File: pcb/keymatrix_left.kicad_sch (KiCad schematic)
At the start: 42 parts, among them SW10 SW_Push, SW11 SW_Push, SW12 SW_Push, SW13 SW_Push, SW14 SW_Push, SW15 SW_Push, SW16 SW_Push, SW17 SW_Push, SW18 SW_Push, SW19 SW_Push, SW2 SW_Push, SW20 SW_Push, SW21 SW_Push, SW22 SW_Push, SW3 SW_Push, SW4 SW_Push, SW5 SW_Push, SW6 SW_Push, SW7 SW_Push, SW8 SW_Push, SW9 SW_Push

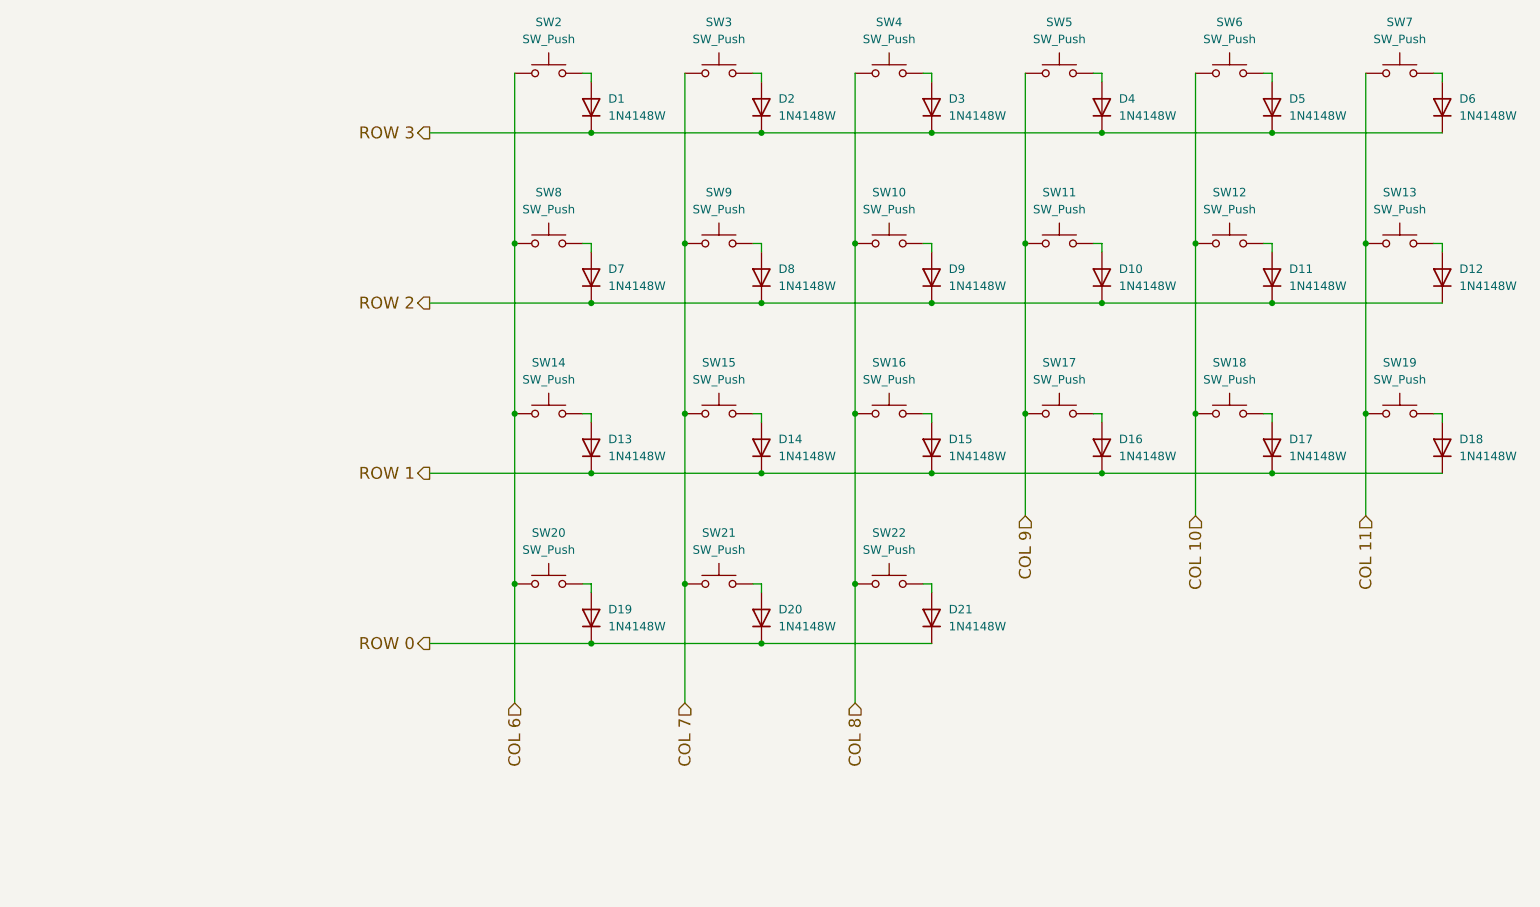
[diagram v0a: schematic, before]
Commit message: update everything
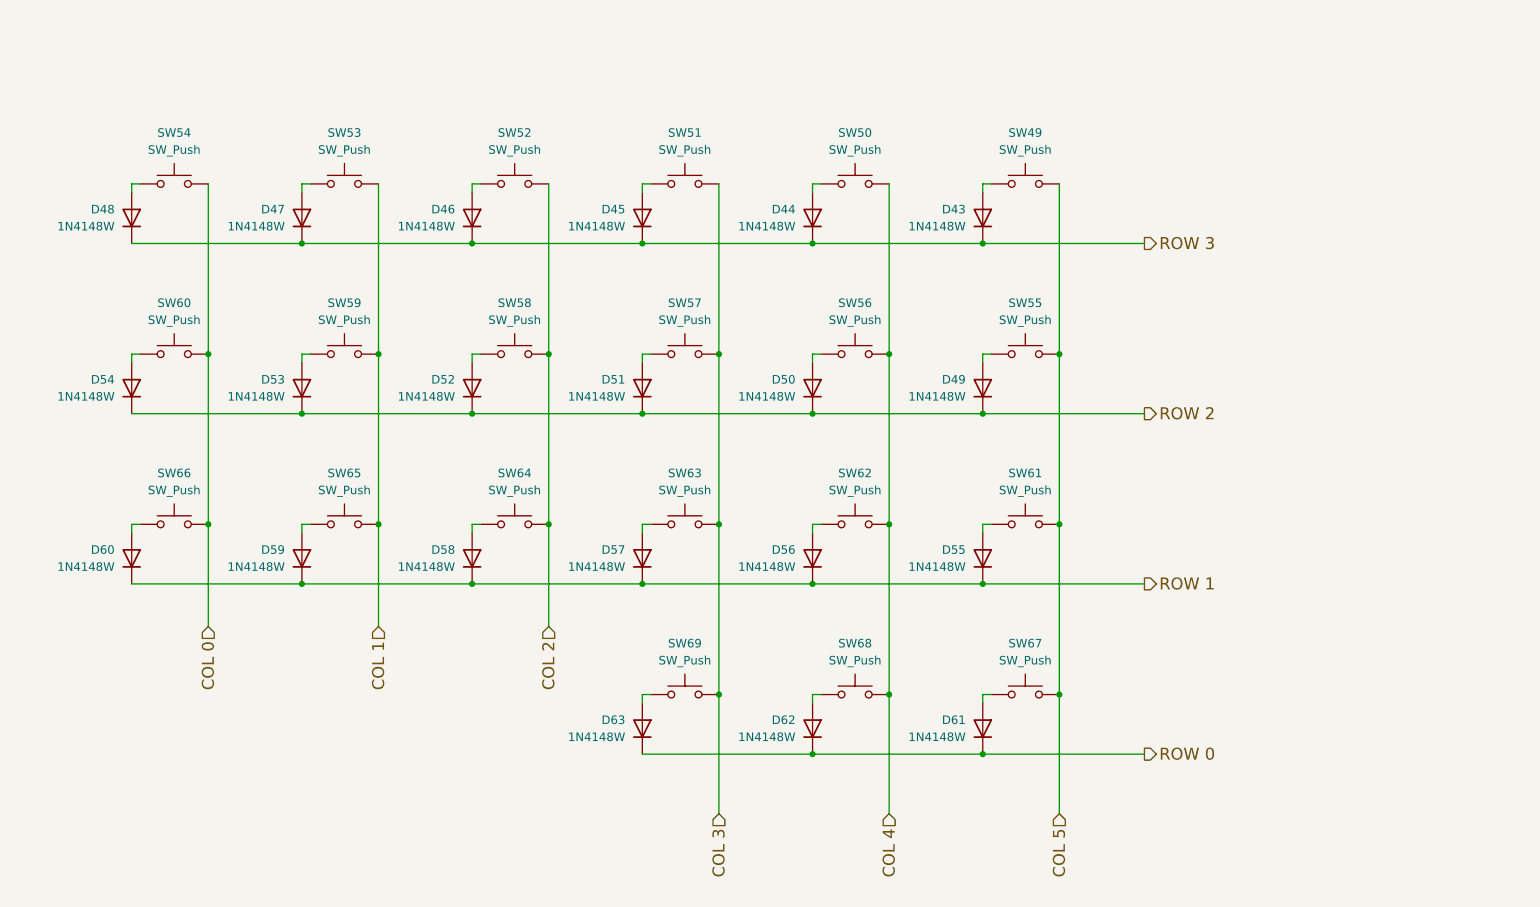
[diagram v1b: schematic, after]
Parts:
- removed D1, D10, D11, D12, D13, D14, D15, D16, D17, D18, D19, D2, D20, D21, D3, D4, D5, D6, D7, D8, D9: 1N4148W, Diode_SMD:D_SOD-123, symbol Diode:1N4148W
- removed SW10, SW11, SW12, SW13, SW14, SW15, SW16, SW17, SW18, SW19, SW2, SW20, SW21, SW22, SW3, SW4, SW5, SW6, SW7, SW8, SW9: SW_Push, kbd:keyswitch_choc12_hotswap_1u, symbol Switch:SW_Push
- added D43, D44, D45, D46, D47, D48, D49, D50, D51, D52, D53, D54, D55, D56, D57, D58, D59, D60, D61, D62, D63: 1N4148W, Diode_SMD:D_SOD-123, symbol Diode:1N4148W
- added SW49, SW50, SW51, SW52, SW53, SW54, SW55, SW56, SW57, SW58, SW59, SW60, SW61, SW62, SW63, SW64, SW65, SW66, SW67, SW68, SW69: SW_Push, kbd:keyswitch_choc12_hotswap_1u, symbol Switch:SW_Push
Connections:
- net ROW 0: now also D61.1 (K), D62.1 (K), D63.1 (K)
- net ROW 1: now also D55.1 (K), D56.1 (K), D57.1 (K), D58.1 (K), D59.1 (K), D60.1 (K)
- net ROW 2: now also D49.1 (K), D50.1 (K), D51.1 (K), D52.1 (K), D53.1 (K), D54.1 (K)
- net ROW 3: now also D43.1 (K), D44.1 (K), D45.1 (K), D46.1 (K), D47.1 (K), D48.1 (K)
- new net: D59.2 (A), SW65.2
- new net: D57.2 (A), SW63.2
- new net: D49.2 (A), SW55.2
- new net: D54.2 (A), SW60.2
- new net: D58.2 (A), SW64.2
- new net: D51.2 (A), SW57.2
- new net: D45.2 (A), SW51.2
- new net: D48.2 (A), SW54.2
- new net: D50.2 (A), SW56.2
- new net: D63.2 (A), SW69.2
- new net: D60.2 (A), SW66.2
- new net: D46.2 (A), SW52.2
- new net: D52.2 (A), SW58.2
- new net: D56.2 (A), SW62.2
- new net: D44.2 (A), SW50.2
- new net: D55.2 (A), SW61.2
- new net: D61.2 (A), SW67.2
- new net: D43.2 (A), SW49.2
- new net: D62.2 (A), SW68.2
- new net: D47.2 (A), SW53.2
- new net: D53.2 (A), SW59.2
- new net COL 0: SW54.1, SW60.1, SW66.1
- new net COL 1: SW53.1, SW59.1, SW65.1
- new net COL 2: SW52.1, SW58.1, SW64.1
- new net COL 3: SW51.1, SW57.1, SW63.1, SW69.1
- new net COL 4: SW50.1, SW56.1, SW62.1, SW68.1
- new net COL 5: SW49.1, SW55.1, SW61.1, SW67.1
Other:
- company: (none) -> Dylan DiBeneditto

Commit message: finished routing second half
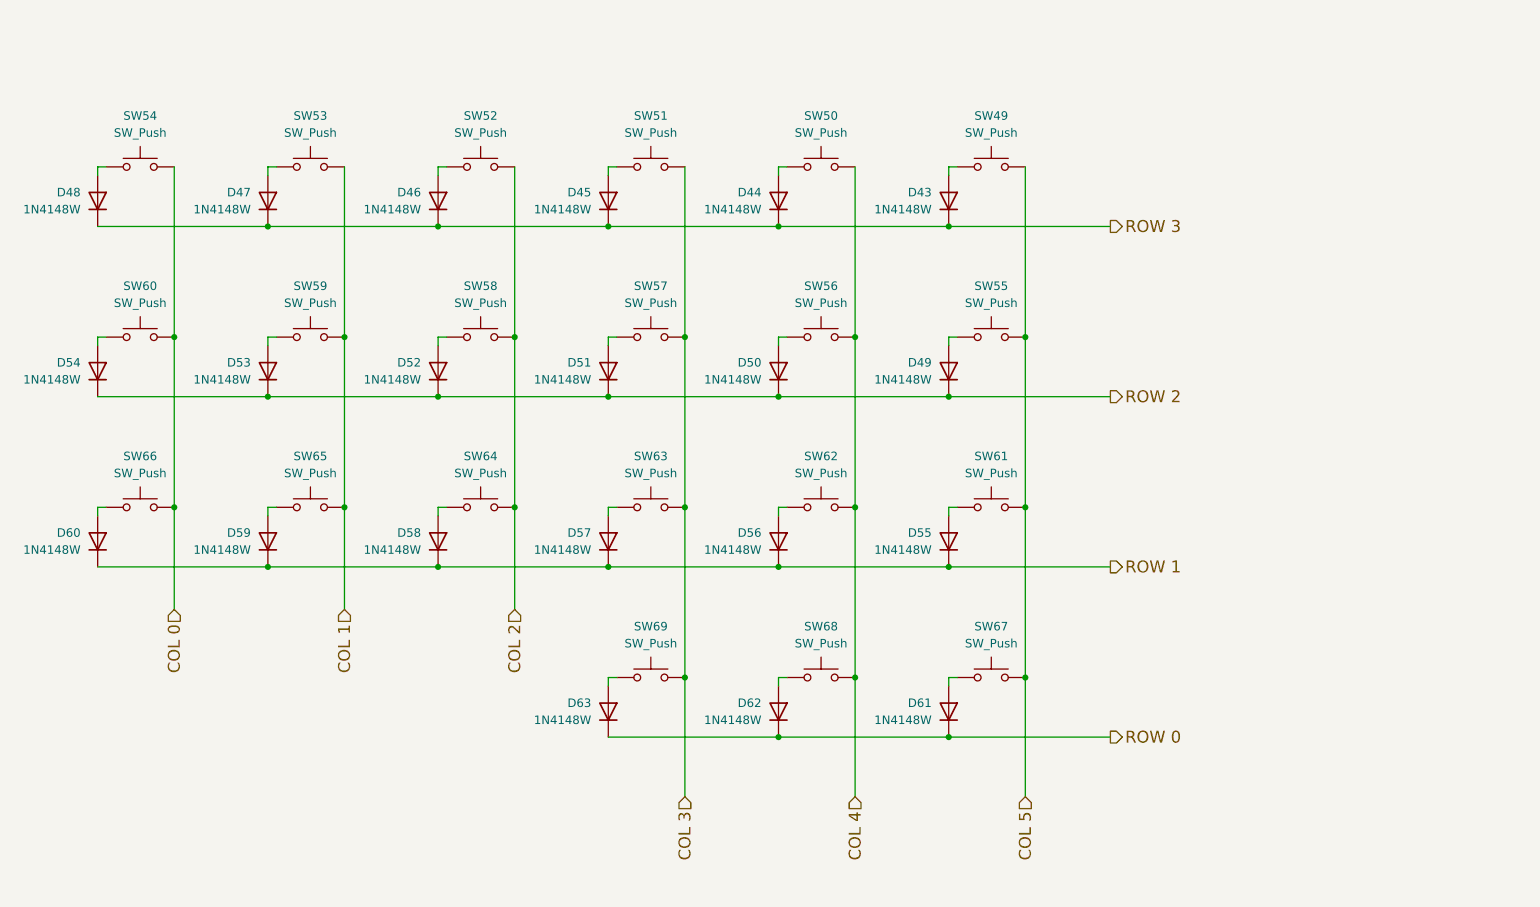
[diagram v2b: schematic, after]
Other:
- moved on the sheet: D43, D44, D45, D46, D47, D48, D49, D50, D51, D52, D53, D54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
